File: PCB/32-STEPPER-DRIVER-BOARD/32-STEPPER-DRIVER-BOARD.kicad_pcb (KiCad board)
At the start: 4 copper layers, 115 x 102.8 mm, 348 parts, among them J1 MEC2-30-01-X-TH1-NP-WT, J2 MEC2-30-01-X-TH1-NP-WT, J3 MEC2-30-01-X-TH1-NP-WT, J4 MEC2-30-01-X-TH1-NP-WT, J5 IPS1-125-01-S-D, J6 UMPT-06-01-X-RA-WT-P-X, U1 74HC595, U10 74HC595, U11 74HC595, U12 74HC595, U13 74HC595, U14 74HC595, U15 74HC595, U16 74HC595, U17 74HC595, U18 74HC595, U19 74HC595, U2 74HC595, U20 74HC595, U21 74HC595, U3 74HC595, U4 74HC595, U5 74HC595, U6 74HC595, U7 74HC595, U9 74HC595

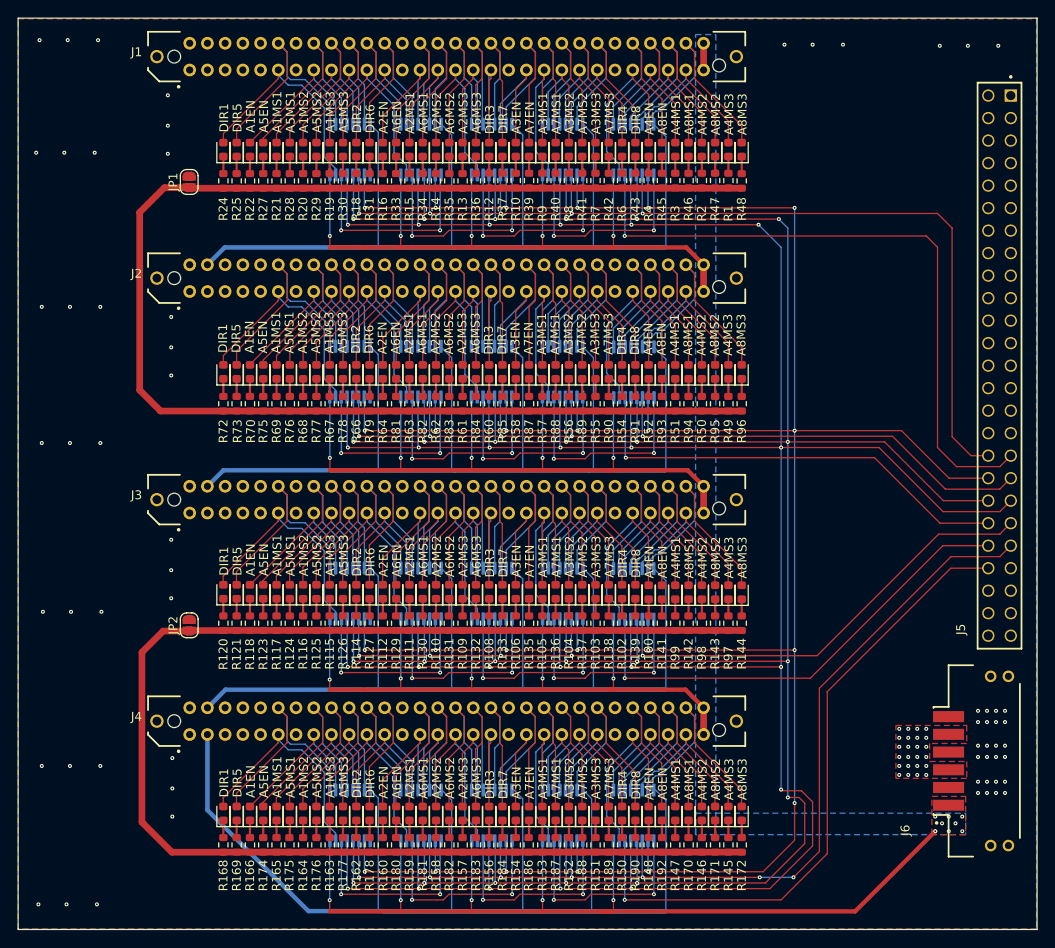
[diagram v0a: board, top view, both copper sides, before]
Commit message: Final checks for 32-stepper driver
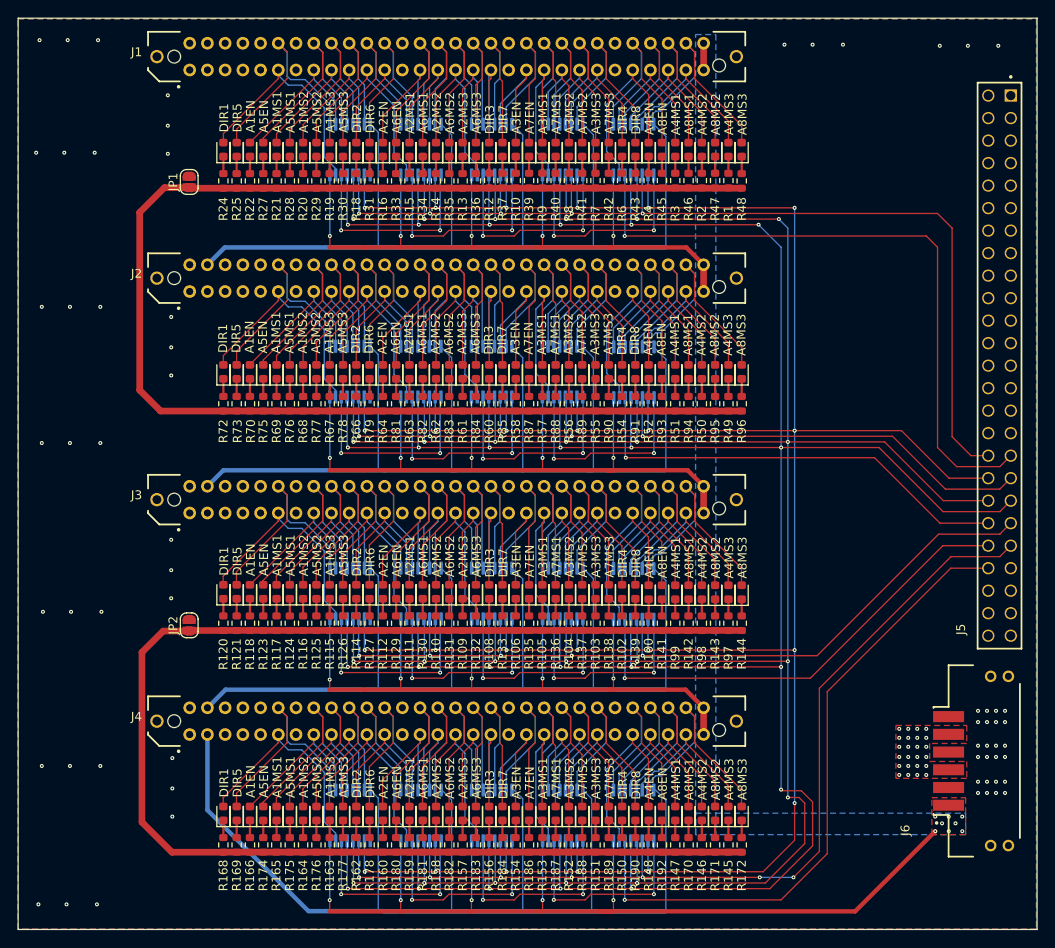
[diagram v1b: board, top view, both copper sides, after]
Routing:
- added copper zone on B.Cu, net GND
- added copper zone on In1.Cu, net GND
